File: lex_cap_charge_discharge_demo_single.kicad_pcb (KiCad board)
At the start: 2 copper layers, 38 x 33.5 mm, 8 parts, among them J1 +5V, J2 GND, SW1 charge, SW2 discharge

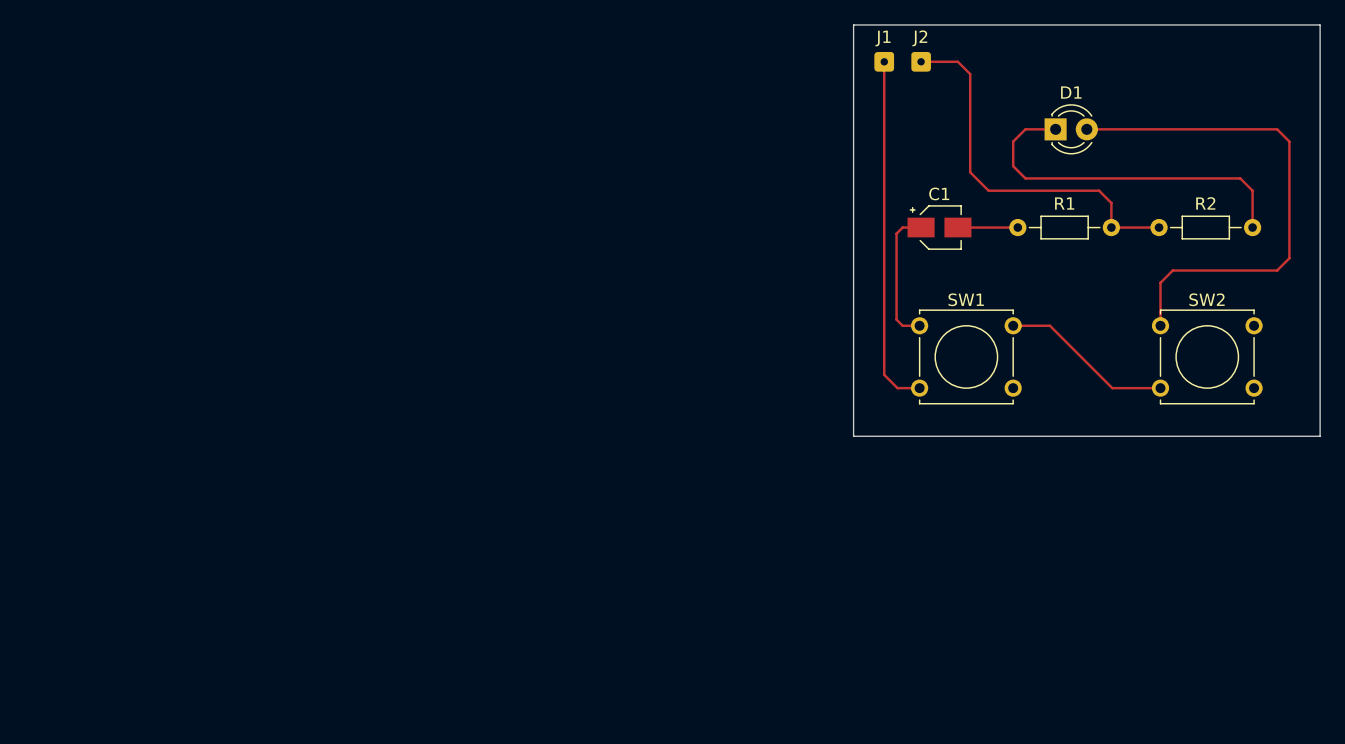
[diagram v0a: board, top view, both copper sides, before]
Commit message: Tweak R vals
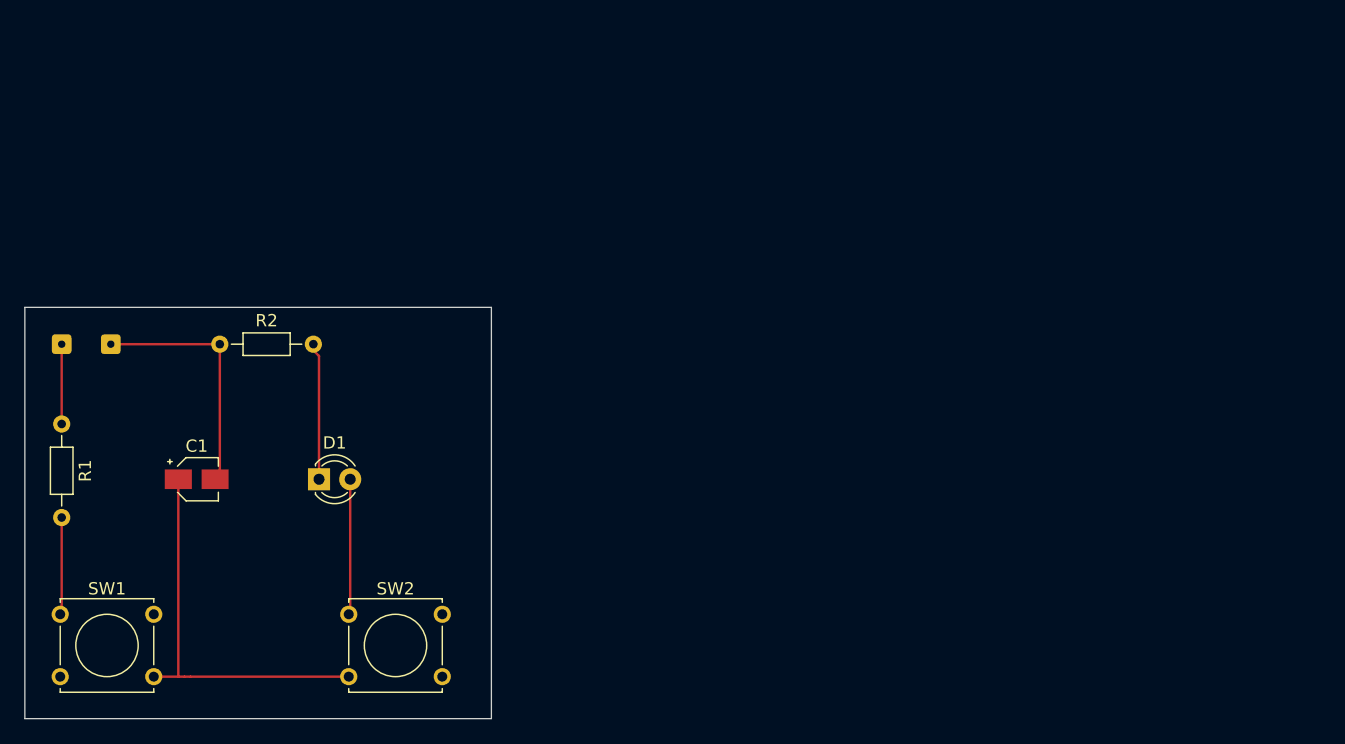
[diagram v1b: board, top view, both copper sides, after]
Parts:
- R1: value 400K -> 10K
- R2: value 470 -> 330
- moved R1 79.5 mm to (53.0, 59.5), turned to -90 degrees
- moved R2 77.1 mm to (65.9, 53.0)
- moved SW1 73.8 mm to (52.9, 75.0)
- moved J1 70.8 mm to (53.0, 53.0)
- moved SW2 70.2 mm to (76.4, 75.0)
- moved J2 69.9 mm to (57.0, 53.0)
- moved D1 66.4 mm to (74.0, 64.0)
- moved C1 63.9 mm to (64.0, 64.0)
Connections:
- C1 pad 1: Net-(SW1-A) -> Net-(SW1-B)
- C1 pad 2: Net-(C1-Pad2) -> GND
- R1 pad 1: Net-(C1-Pad2) -> +5V
- R1 pad 2: GND -> Net-(SW1-A)
- SW1 pad 2: +5V -> Net-(SW1-B)
- SW2 pad 2: Net-(SW1-A) -> Net-(SW1-B)
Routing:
- net Net-(SW1-B): track 0.00 -> 32.0 mm
- net Net-(D1-A): track 41.2 -> 11.0 mm
- net +5V: track 28.8 -> 6.50 mm
- net Net-(D1-K): track 29.2 -> 11.2 mm
- net Net-(SW1-A): track 25.4 -> 7.93 mm
- net GND: track 30.8 -> 20.0 mm
- net Net-(C1-Pad2): track 4.88 -> 0.00 mm
